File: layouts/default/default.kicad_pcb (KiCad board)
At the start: 2 copper layers, 60 x 60 mm, 37 parts

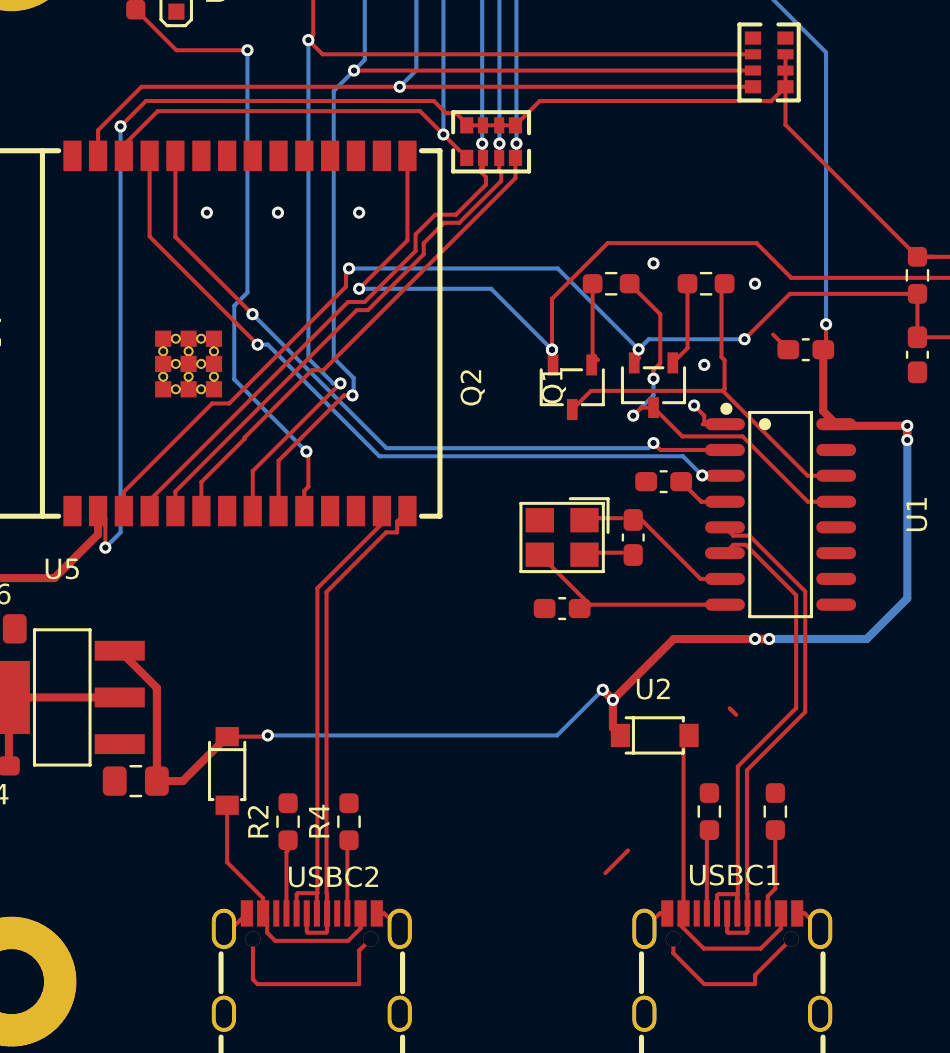
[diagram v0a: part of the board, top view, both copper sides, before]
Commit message: Cleanupy
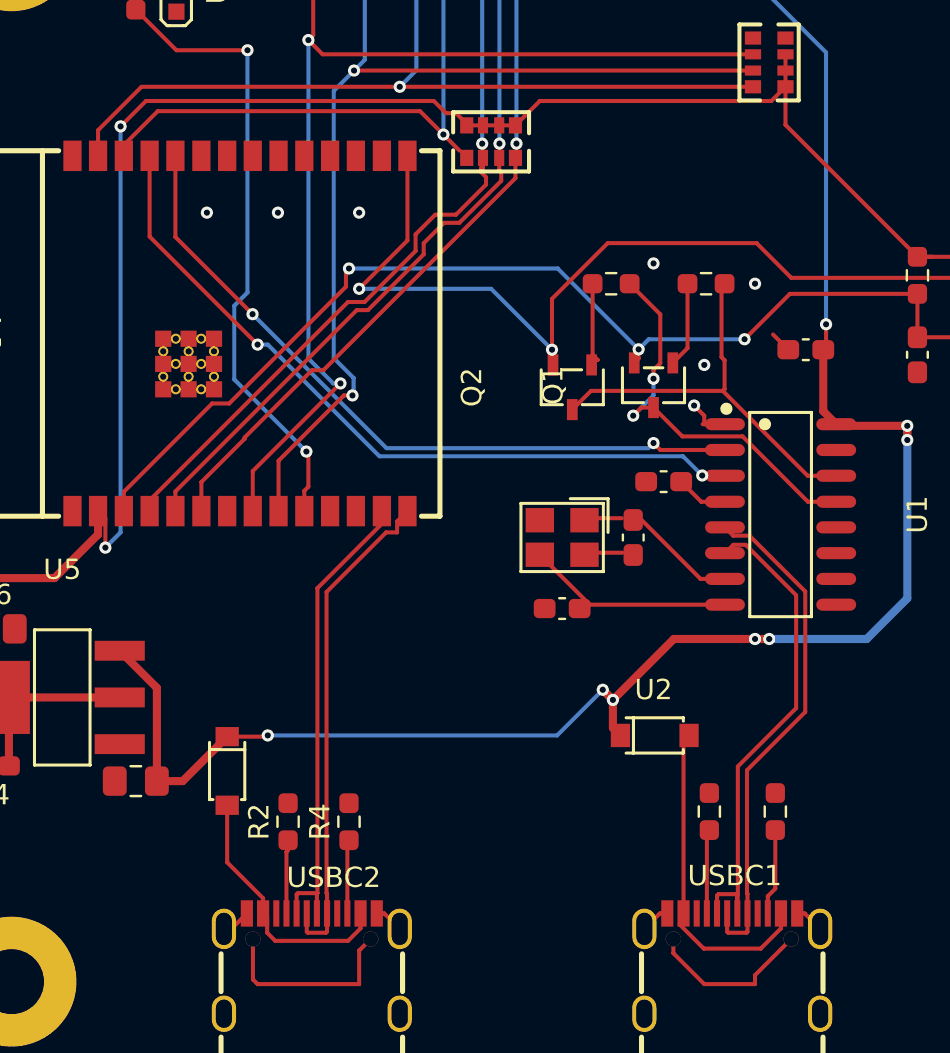
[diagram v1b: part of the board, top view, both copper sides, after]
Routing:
- net cc1_r_debug-A5: track 6.20 -> 3.98 mm
- net diode_debug-VBUS: track 16.1 -> 15.1 mm
- net esp32-D_N: track 23.1 -> 22.5 mm
- net IO4: track 39.0 -> 38.5 mm
- net IO3: track 30.6 -> 30.1 mm
- net boot_pullup-E: track 49.7 -> 49.6 mm, vias 3 -> 2
